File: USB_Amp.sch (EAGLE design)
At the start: 184 parts, among them CON1 USB-C, CON2 PIC32_CON, CON3 VOLUEME, CON4 SWD, IC1 3.3V, IC10 1.8V, IC11 STM32G031F, IC12 +5V, IC13 3.3V, IC2 PIC32MZEF, IC3 +12V, IC4 +5V, IC5 TAS2780, IC6 1.8V, IC7 +12V, IC8 +5V, IC9 TAS2780, X1 24.576MHz, X2 22.5792MHz, X3 12MHz

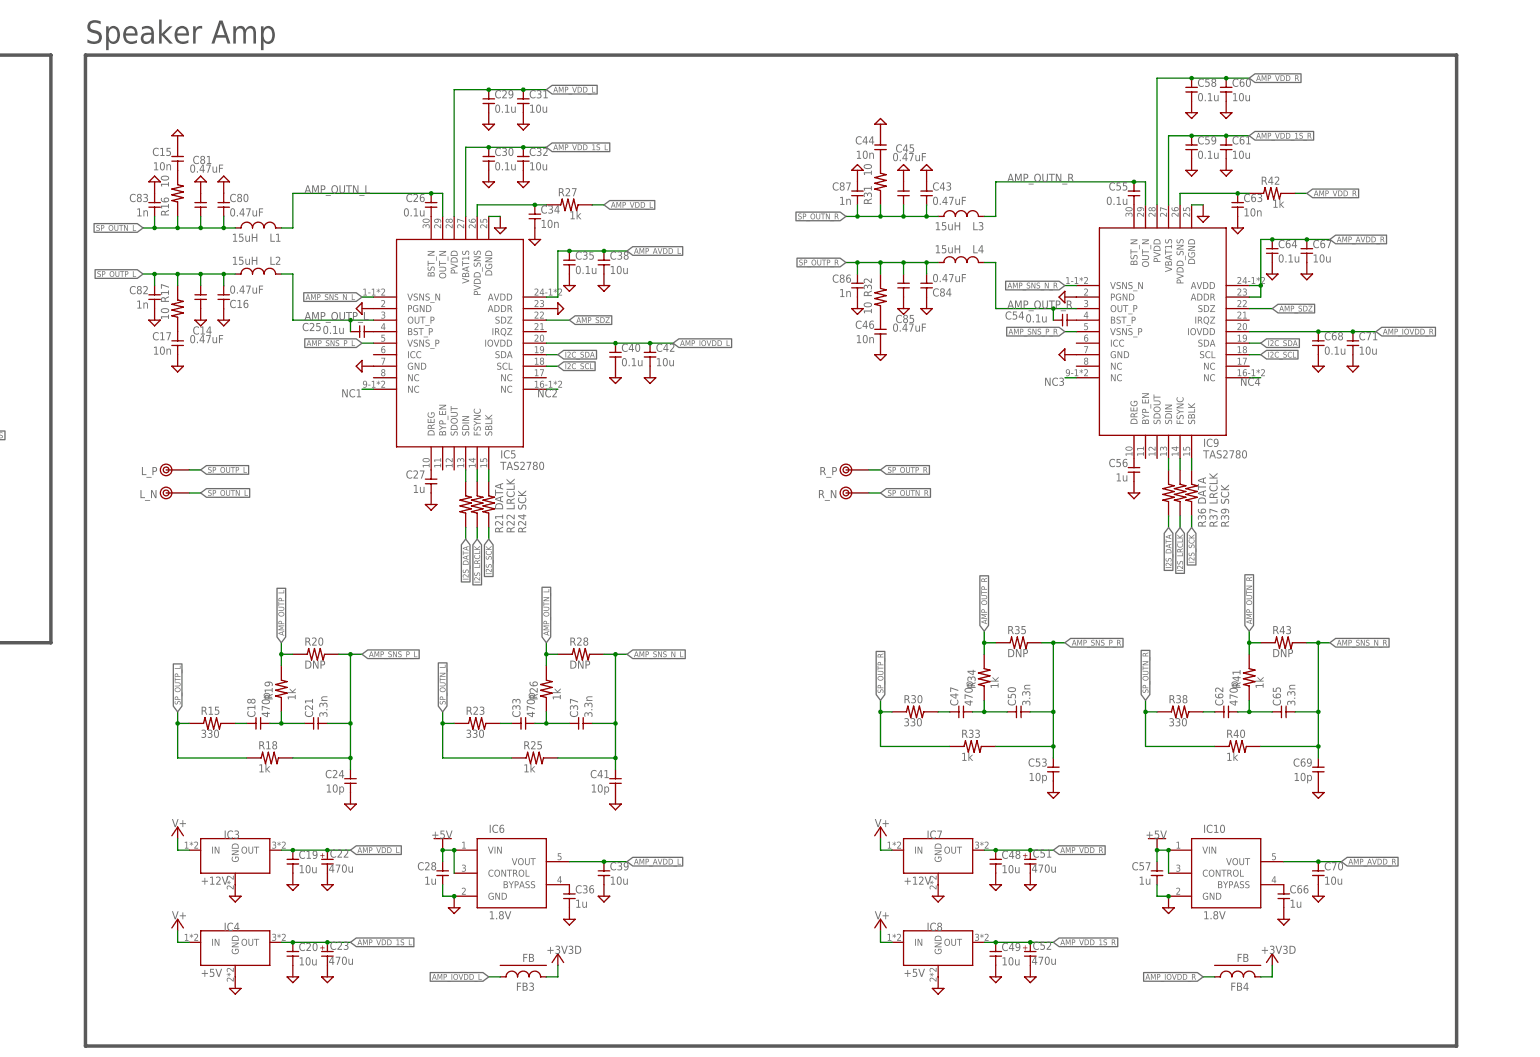
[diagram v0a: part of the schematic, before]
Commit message: TAS2770
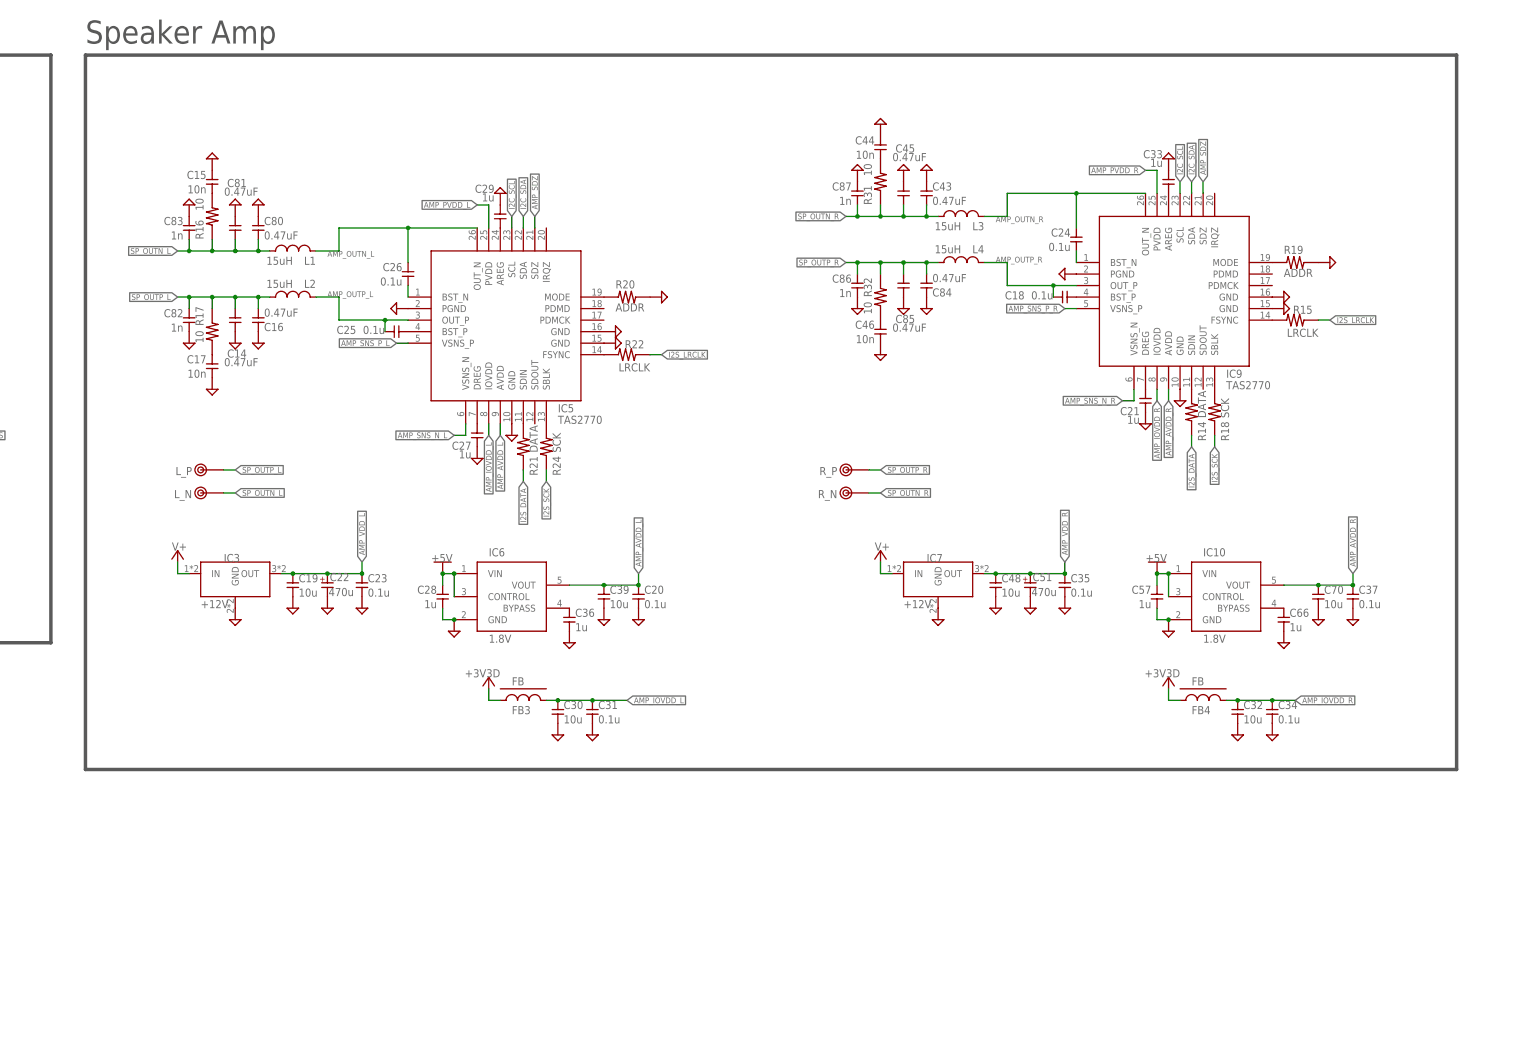
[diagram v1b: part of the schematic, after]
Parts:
- removed C38, C42, C60, C61, C67, C71: 10u, my_rcl:C-2012
- removed C40, C54, C55, C58, C59, C64, C68: 0.1u, my_rcl:C-1608
- removed C41, C53, C69: 10p, my_rcl:C-1608
- removed C47, C62: 470p, my_rcl:C-1608
- removed C49: 10u, my_rcl:C-3216
- removed C50, C65: 3.3n, my_rcl:C-1608
- removed C52: 470u, my_rcl:CPOLE5-10-DUAL
- removed C56: 1u, my_rcl:C-1608
- removed C63: 10n, my_rcl:C-1608
- removed IC4, IC8: +5V, my_ic:78X-3
- removed R23, R30, R38: 330, my_rcl:R-1608
- removed R25, R26, R27, R33, R34, R40, R41, R42: 1k, my_rcl:R-1608
- removed R28, R35, R43: DNP, my_rcl:R-1608
- removed R36: DATA, my_rcl:R-1608J
- removed R37: LRCLK, my_rcl:R-1608J
- removed R39: SCK, my_rcl:R-1608J
- added R14: DATA, my_rcl:R-1608J
- C16, C43, C80, C84: device my_rcl:C-5 -> my_rcl:C-5W
- C18: value 470p -> 0.1u
- C20: value 10u -> 0.1u; device my_rcl:C-3216 -> my_rcl:C-1608
- C21: value 3.3n -> 1u
- C23: value 470u -> 0.1u; device my_rcl:CPOLE5-10-DUAL -> my_rcl:C-1608
- C24: value 10p -> 0.1u
- C29: value 0.1u -> 1u
- C30: value 0.1u -> 10u; device my_rcl:C-1608 -> my_rcl:C-2012
- C31: value 10u -> 0.1u; device my_rcl:C-2012 -> my_rcl:C-1608
- C33: value 470p -> 1u
- C34: value 10n -> 0.1u
- C37: value 3.3n -> 0.1u
- IC5, IC9: value TAS2780 -> TAS2770; device my_ic:TAS2780 -> my_ic:TAS2770
- R15: value 330 -> LRCLK; device my_rcl:R-1608 -> my_rcl:R-1608J
- R18: value 1k -> SCK; device my_rcl:R-1608 -> my_rcl:R-1608J
- R19: value 1k -> ADDR
- R20: value DNP -> ADDR
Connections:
- removed net AMP_VDD_1S_L: C20.1, C23.1, C30.1, C32.1, IC4.OUT, IC5.VBAT1S
- removed net AMP_VDD_1S_R: C49.1, C52.1, C59.1, C61.1, IC8.OUT, IC9.VBAT1S
- removed net N$14 (its old number): C34.1, IC5.PVDD_SNS, R27.1
- removed net N$28: IC9.FSYNC, R37.2
- removed net N$29: IC9.SBLK, R39.2
- removed net N$32: C47.2, C50.1, R34.1
- removed net N$33: C47.1, R30.2
- removed net N$34: C62.2, C65.1, R41.1
- removed net N$35: C62.1, R38.2
- removed net NC1: IC5.NC@2
- removed net NC2: IC5.NC@3
- removed net NC3: IC9.NC@2
- removed net NC4: IC9.NC@3
- new net AMP_PVDD_L: IC5.PVDD
- new net AMP_PVDD_R: IC9.PVDD
- new net N$18: C29.2, IC5.AREG
- net AMP_AVDD_L: now also C20.1; no longer C35.1, C38.1
- net AMP_AVDD_R: now also C37.1; no longer C64.1, C67.1, IC9.ADDR
- net AMP_IOVDD_L: now also C30.1, C31.1; no longer C40.1, C42.1
- net AMP_IOVDD_R: now also C32.1, C34.1; no longer C68.1, C71.1
- net AMP_OUTN_L: no longer R26.2, R28.1
- net AMP_OUTN_R: now also C24.1; no longer C55.1, R41.2, R43.1
- net AMP_OUTP_L: no longer R19.2, R20.1
- net AMP_OUTP_R: now also C18.2; no longer C54.2, R34.2, R35.1
- net AMP_SNS_N_L: no longer C37.2, C41.1, R25.2, R28.2
- net AMP_SNS_N_R: no longer C65.2, C69.1, R40.2, R43.2
- net AMP_SNS_P_L: no longer C21.2, C24.1, R18.2, R20.2
- net AMP_SNS_P_R: no longer C50.2, C53.1, R33.2, R35.2
- net AMP_VDD_L: now also C23.1; no longer C29.1, C31.1, IC5.PVDD, R27.2
- net AMP_VDD_R: now also C35.1; no longer C58.1, C60.1, IC9.PVDD, R42.2
- net GND: now also C21.2, C29.1, C33.1, C37.2, IC5.GND@2, IC5.GND@3, IC5.PGND, IC9.GND@2, IC9.GND@3, IC9.PGND, R19.2, R20.2; no longer C24.2, C29.2, C38.2, C40.2, C41.2, C42.2, C49.2, C52.2, C53.2, C56.2, C58.2, C59.2, C60.2, C61.2, C63.2, C64.2, C67.2, C68.2, C69.2, C71.2, IC4.GND, IC5.ADDR, IC5.DGND, IC5.PGND@1, IC8.GND, IC9.DGND, IC9.PGND@1
- net I2S_DATA: now also R14.1; no longer R36.1
- net I2S_LRCLK: now also R15.1; no longer R37.1
- net I2S_SCK: now also R18.1; no longer R39.1
- net N$10: now also IC9.SDIN, R14.2; no longer C33.2, C37.1, R26.1
- net N$13: now also IC9.SBLK, R18.2; no longer C18.2, C21.1, R19.1
- net N$19: now also IC9.FSYNC, R15.2; no longer C33.1, R23.2
- net N$20: now also C21.1, IC9.DREG; no longer C18.1, R15.2
- net N$23: now also C18.1, IC9.BST_P; no longer C55.2, IC9.BST_N
- net N$24: now also C24.2, IC9.BST_N; no longer C54.1, IC9.BST_P
- net N$25: now also C33.2, IC9.AREG; no longer C63.1, IC9.PVDD_SNS, R42.1
- net N$26: now also IC9.MODE, R19.1; no longer C56.1, IC9.DREG
- net N$27: now also IC5.MODE, R20.1; no longer IC9.SDIN, R36.2
- net SP_OUTN_L: no longer R23.1, R25.1
- net SP_OUTN_R: no longer R38.1, R40.1
- net SP_OUTP_L: no longer R15.1, R18.1
- net SP_OUTP_R: no longer R30.1, R33.1
- net V+: no longer IC4.IN, IC8.IN
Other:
- moved on the sheet: C14, C15, C16, C17, C18, C19, C20, C21, C22, C24, C25, C26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
